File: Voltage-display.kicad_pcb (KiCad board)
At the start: 2 copper layers, 39 parts, among them IC1 TC7107ACPL, J1 Conn_01x02, J2 Conn_01x02, Q1 DMP2035UQ-7, SW1 BD01, U2 PAMC3311QDWERQ1, U3 TC7660SEPA, U4 ADR510ARTZ-REEL7

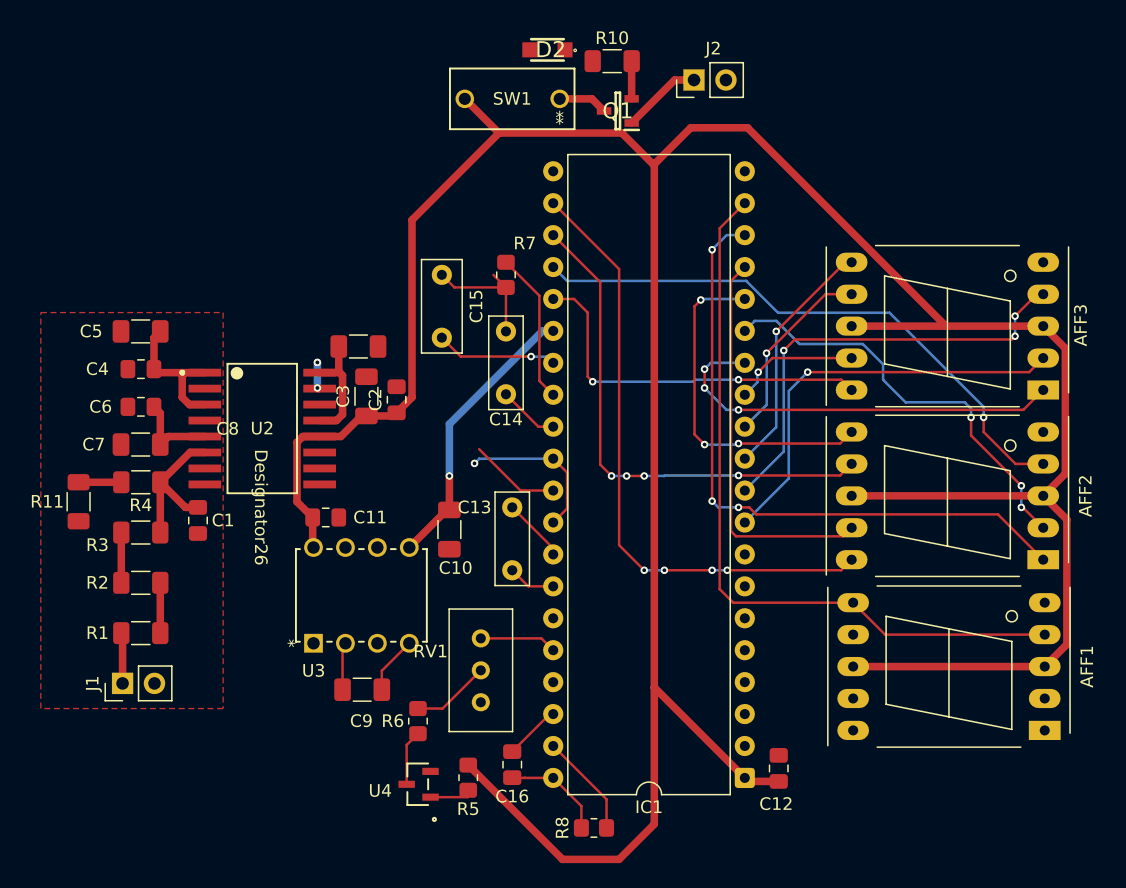
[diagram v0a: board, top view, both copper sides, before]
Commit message: Update schematic
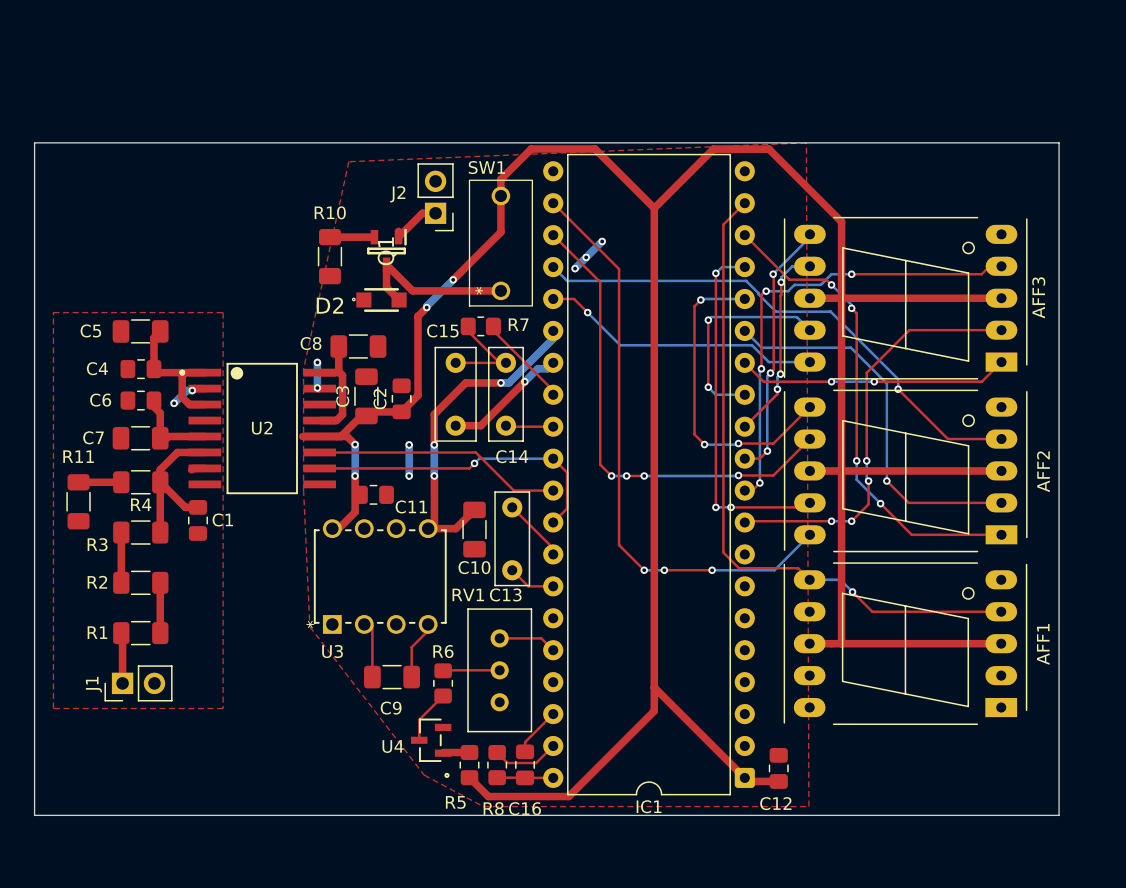
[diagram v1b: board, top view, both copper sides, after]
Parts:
- moved R10 27.3 mm to (143.5, 72.0), turned to 90 degrees
- moved D2 23.9 mm to (147.6, 75.5), turned to 0 degrees
- moved J2 23.1 mm to (151.9, 68.6), turned to 180 degrees
- moved Q1 21.5 mm to (148.0, 71.6), turned to -90 degrees
- moved SW1 16.0 mm to (157.1, 74.8), turned to 90 degrees
- moved R8 9.18 mm to (156.8, 112.5), turned to -90 degrees
- moved C15 7.09 mm to (153.5, 80.5)
- moved R7 4.56 mm to (155.5, 77.6), turned to 180 degrees
- moved C11 4.20 mm to (147.0, 91.0)
- moved AFF3 3.99 mm to (196.9, 80.4)
- moved AFF1 3.91 mm to (196.9, 107.9)
- moved AFF2 3.87 mm to (196.9, 94.2)
- moved U4 3.64 mm to (151.5, 110.5)
- moved R6 3.61 mm to (152.5, 106.0)
- moved C9 2.58 mm to (148.4, 105.5)
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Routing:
- net +5V: track 251.5 -> 223.9 mm, vias 0 -> 4
- net /TC7107_Display/E3: track 51.4 -> 38.2 mm, vias 3 -> 4
- net /TC7107_Display/AMC_OUTP: track 7.26 -> 19.8 mm
- net /TC7107_Display/AMC_OUTN: track 12.6 -> 24.9 mm
- net /TC7107_Display/E2: track 33.2 -> 21.7 mm, vias 3 -> 2
- net Net-(D2-A2): track 3.92 -> 13.2 mm
- net /TC7107_Display/G2: track 29.9 -> 22.5 mm, vias 2 -> 1
- net /TC7107_Display/F2: track 10.1 -> 17.1 mm, vias 1 -> 2
- net /TC7107_Display/AB4: track 58.9 -> 52.5 mm, vias 0 -> 1
- net GND: track 2.23 -> 7.75 mm, vias 2 -> 7
- net /TC7107_Display/V_BUFF: track 12.1 -> 7.04 mm
- net /TC7107_Display/C3: track 46.6 -> 41.8 mm
- net HV-: track 0.00 -> 4.02 mm, vias 0 -> 2
- net /TC7107_Display/OSC1: track 8.20 -> 4.47 mm
- net /TC7107_Display/-5V: track 22.5 -> 25.5 mm, vias 1 -> 3
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- added copper zone on F.Cu, net GND
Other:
- board outline added: 81.5 x 53.5 mm
